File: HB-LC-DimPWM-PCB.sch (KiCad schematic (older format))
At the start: 23 parts, among them J1 SWD, J2 12V Input, U1 STM32F103C8Tx, U2 AMS1117-3.3, U3 HomeMatic-sensor, Y1 8MHz

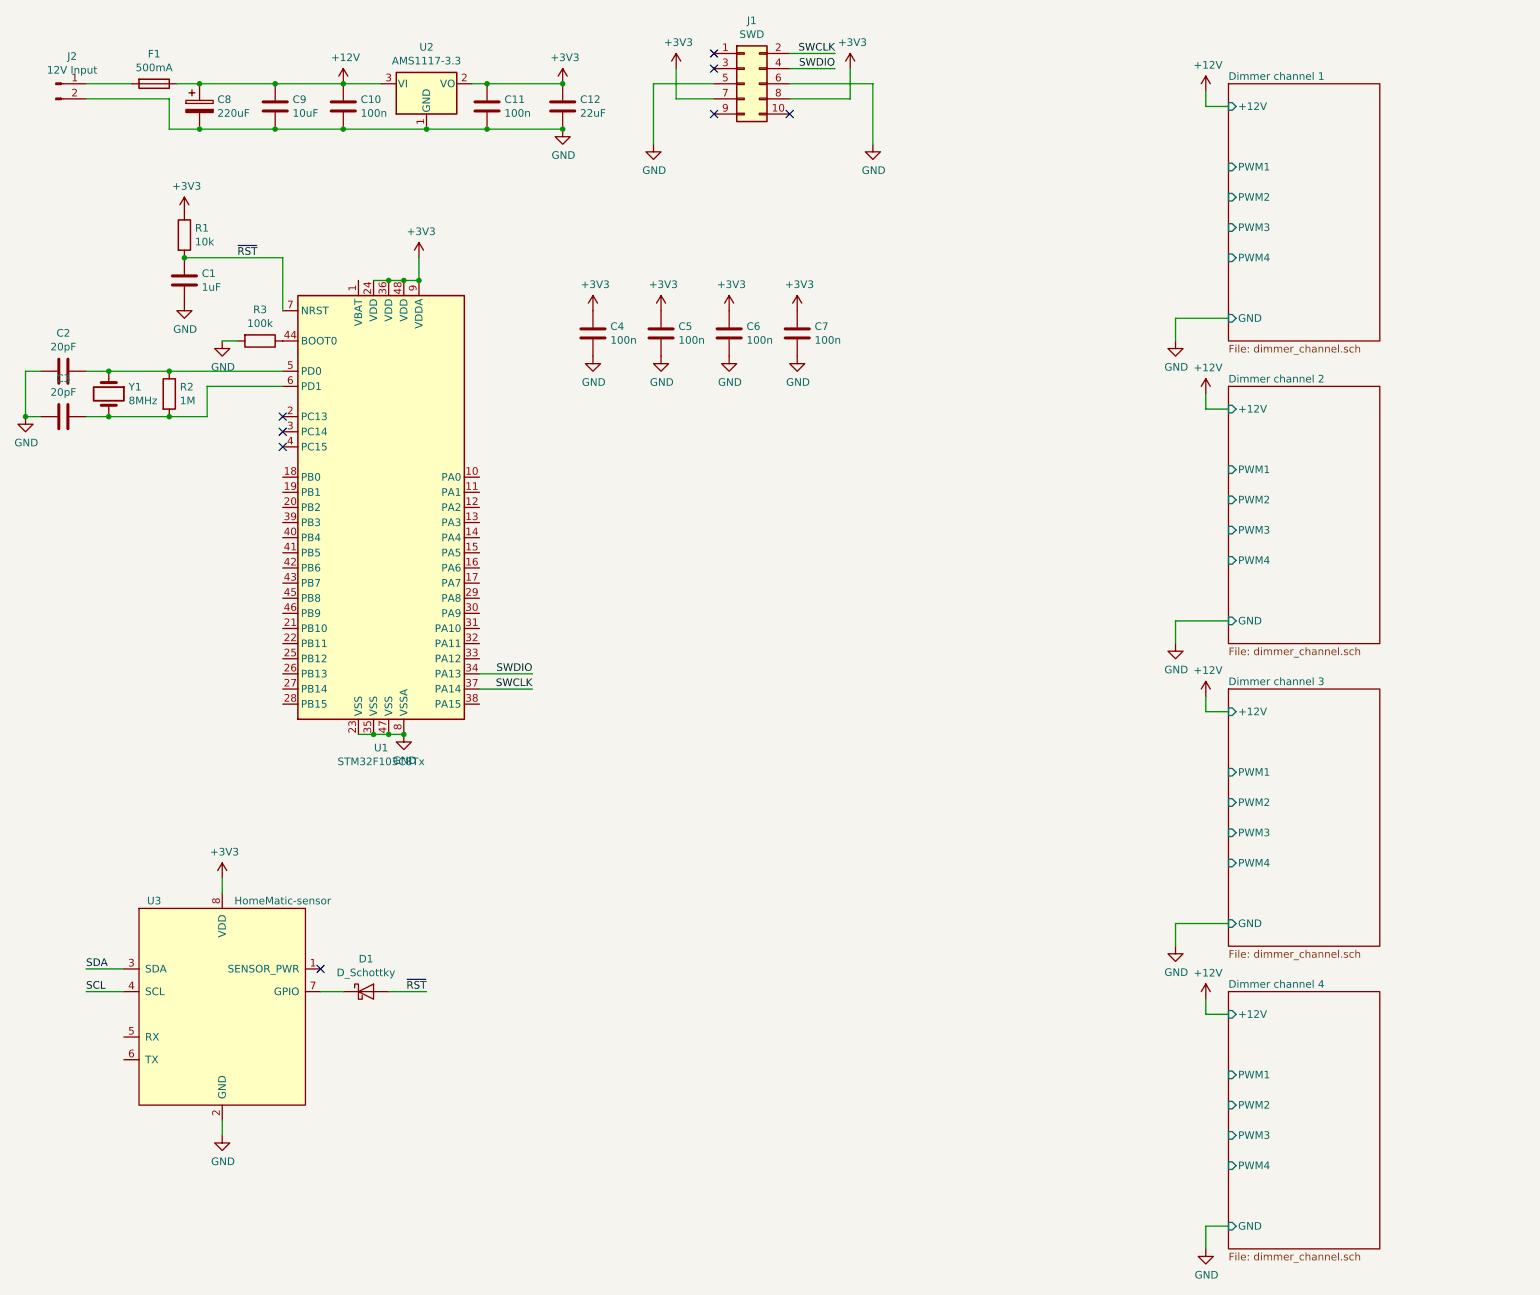
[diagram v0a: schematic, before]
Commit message: Layout board
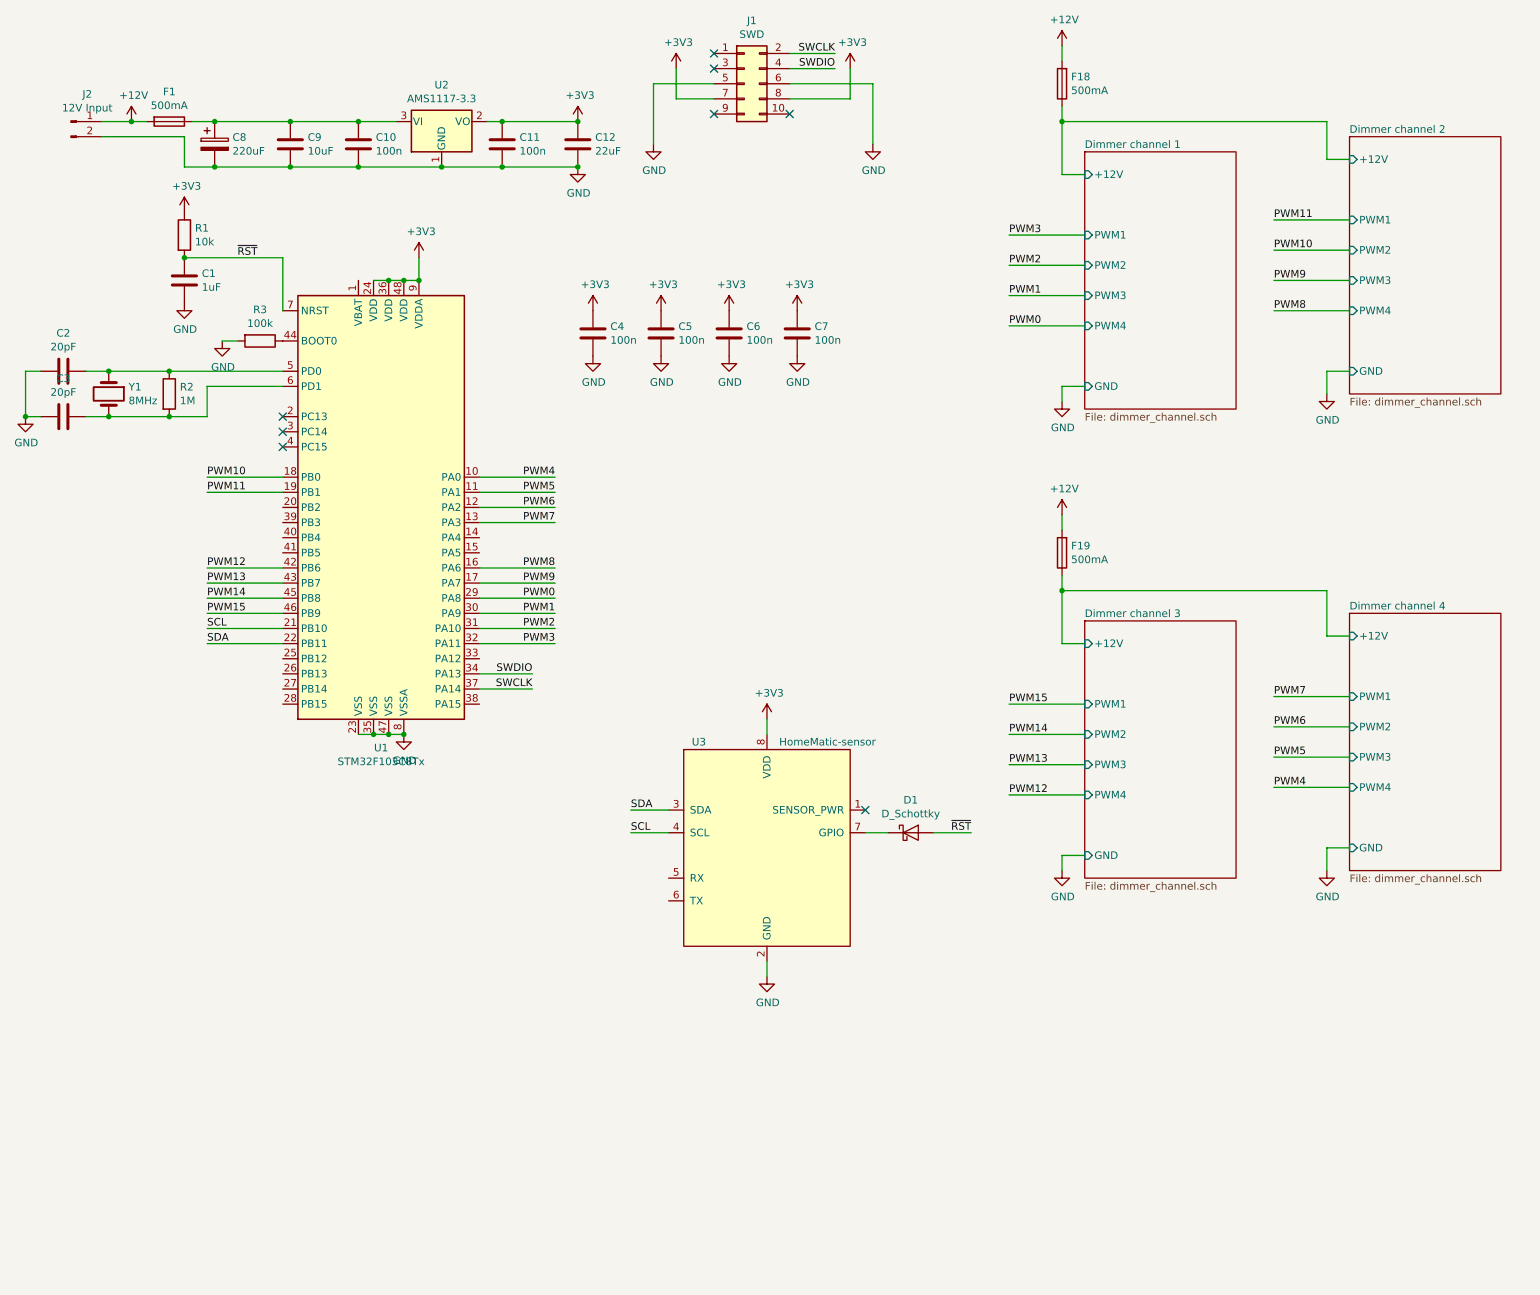
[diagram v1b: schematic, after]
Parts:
- added F18, F19: 500mA, Fuse:Fuse_2512_6332Metric, symbol Device:Fuse
- D1: footprint (none) -> Diode_SMD:D_SOD-123; LCSC (none) -> C8598
- J2: footprint Connector_Phoenix_MC_HighVoltage:PhoenixContact_MC_1,5_2-G-5.08_1x02_P5.08mm_Horizontal -> Connector_Wago_714:Wago_714-162_1x02_P3.50mm_Horizontal
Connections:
- net +12V: now also F1.2, J2.1 (Pin_1), F18.2, F19.2; no longer C10.1, C8.1, C9.1, F1.1, U2.3 (VI)
- net SCL: now also U1.21 (PB10)
- net SDA: now also U1.22 (PB11)
- net PWM4: now reaches U1.10 (PA0)
- net PWM5: now reaches U1.11 (PA1)
- net PWM6: now reaches U1.12 (PA2)
- net PWM7: now reaches U1.13 (PA3)
- net PWM8: now reaches U1.16 (PA6)
- net PWM9: now reaches U1.17 (PA7)
- net PWM10: now reaches U1.18 (PB0)
- net PWM11: now reaches U1.19 (PB1)
- net PWM0: now reaches U1.29 (PA8)
- net PWM1: now reaches U1.30 (PA9)
- net PWM2: now reaches U1.31 (PA10)
- net PWM3: now reaches U1.32 (PA11)
- net PWM12: now reaches U1.42 (PB6)
- net PWM13: now reaches U1.43 (PB7)
- net PWM14: now reaches U1.45 (PB8)
- net PWM15: now reaches U1.46 (PB9)
- new net: C10.1, C8.1, C9.1, F1.1, U2.3 (VI)
- new net Dimmer channel 1/+12V: F18.1
- new net Dimmer channel 3/+12V: F19.1
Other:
- moved on the sheet: C10, C11, C12, C8, C9, D1, F1, J2, U2, U3
